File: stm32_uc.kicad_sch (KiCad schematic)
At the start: 28 parts

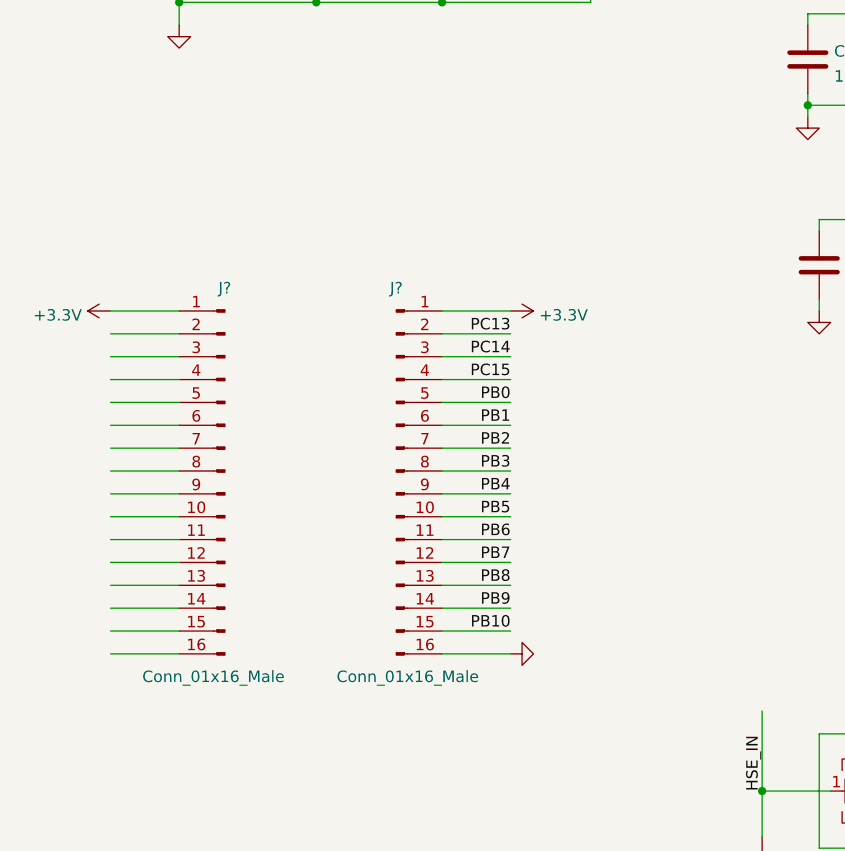
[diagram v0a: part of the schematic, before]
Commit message: finished connectors
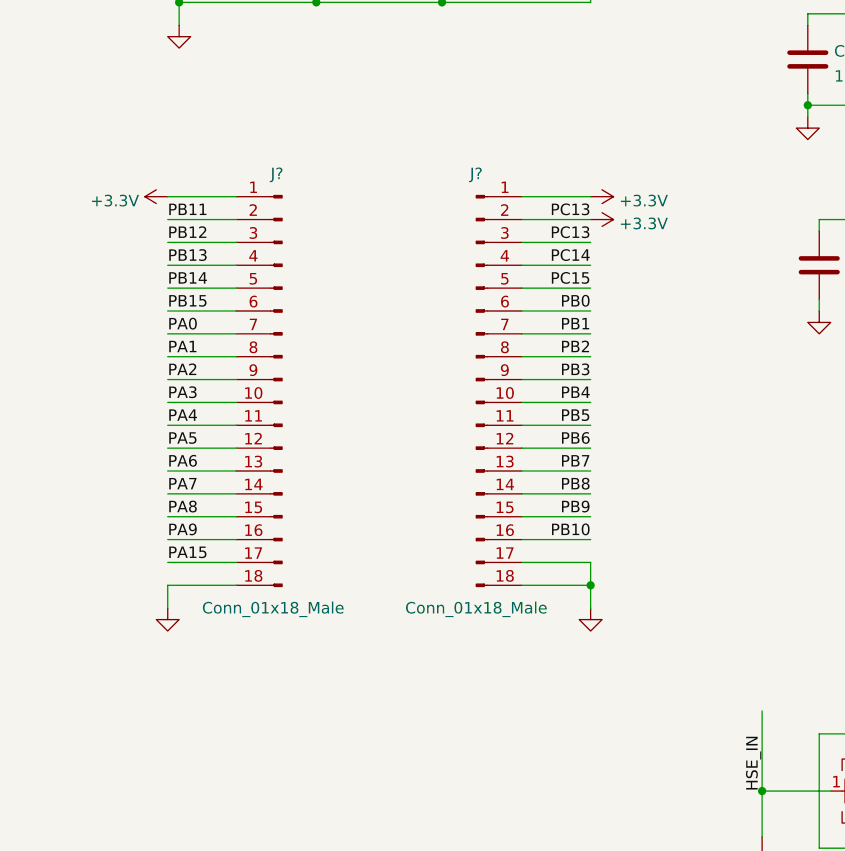
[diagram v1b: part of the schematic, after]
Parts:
- removed J? (x2): Conn_01x16_Male, symbol Connector:Conn_01x16_Male
- added J? (x2): Conn_01x18_Male, symbol Connector:Conn_01x18_Male
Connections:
- net PC13 is gone; now on net +3V3: U?.2 (PC13)
- net +3V3: now also J?.1 (Pin_1), J?.1 (Pin_1), J?.2 (Pin_2), J?.3 (Pin_3)
- net GND: now also J?.17 (Pin_17), J?.18 (Pin_18), J?.18 (Pin_18)
- net PA0: now also J?.7 (Pin_7)
- net PA1: now also J?.8 (Pin_8)
- net PA15: now also J?.17 (Pin_17)
- net PA2: now also J?.9 (Pin_9)
- net PA3: now also J?.10 (Pin_10)
- net PA4: now also J?.11 (Pin_11)
- net PA5: now also J?.12 (Pin_12)
- net PA6: now also J?.13 (Pin_13)
- net PA7: now also J?.14 (Pin_14)
- net PA8: now also J?.15 (Pin_15)
- net PA9: now also J?.16 (Pin_16)
- net PB0: now also J?.6 (Pin_6)
- net PB1: now also J?.7 (Pin_7)
- net PB10: now also J?.16 (Pin_16)
- net PB11: now also J?.2 (Pin_2)
- net PB12: now also J?.3 (Pin_3)
- net PB13: now also J?.4 (Pin_4)
- net PB14: now also J?.5 (Pin_5)
- net PB15: now also J?.6 (Pin_6)
- net PB2: now also J?.8 (Pin_8)
- net PB3: now also J?.9 (Pin_9)
- net PB4: now also J?.10 (Pin_10)
- net PB5: now also J?.11 (Pin_11)
- net PB6: now also J?.12 (Pin_12)
- net PB7: now also J?.13 (Pin_13)
- net PB8: now also J?.14 (Pin_14)
- net PB9: now also J?.15 (Pin_15)
- net PC14: now also J?.4 (Pin_4)
- net PC15: now also J?.5 (Pin_5)

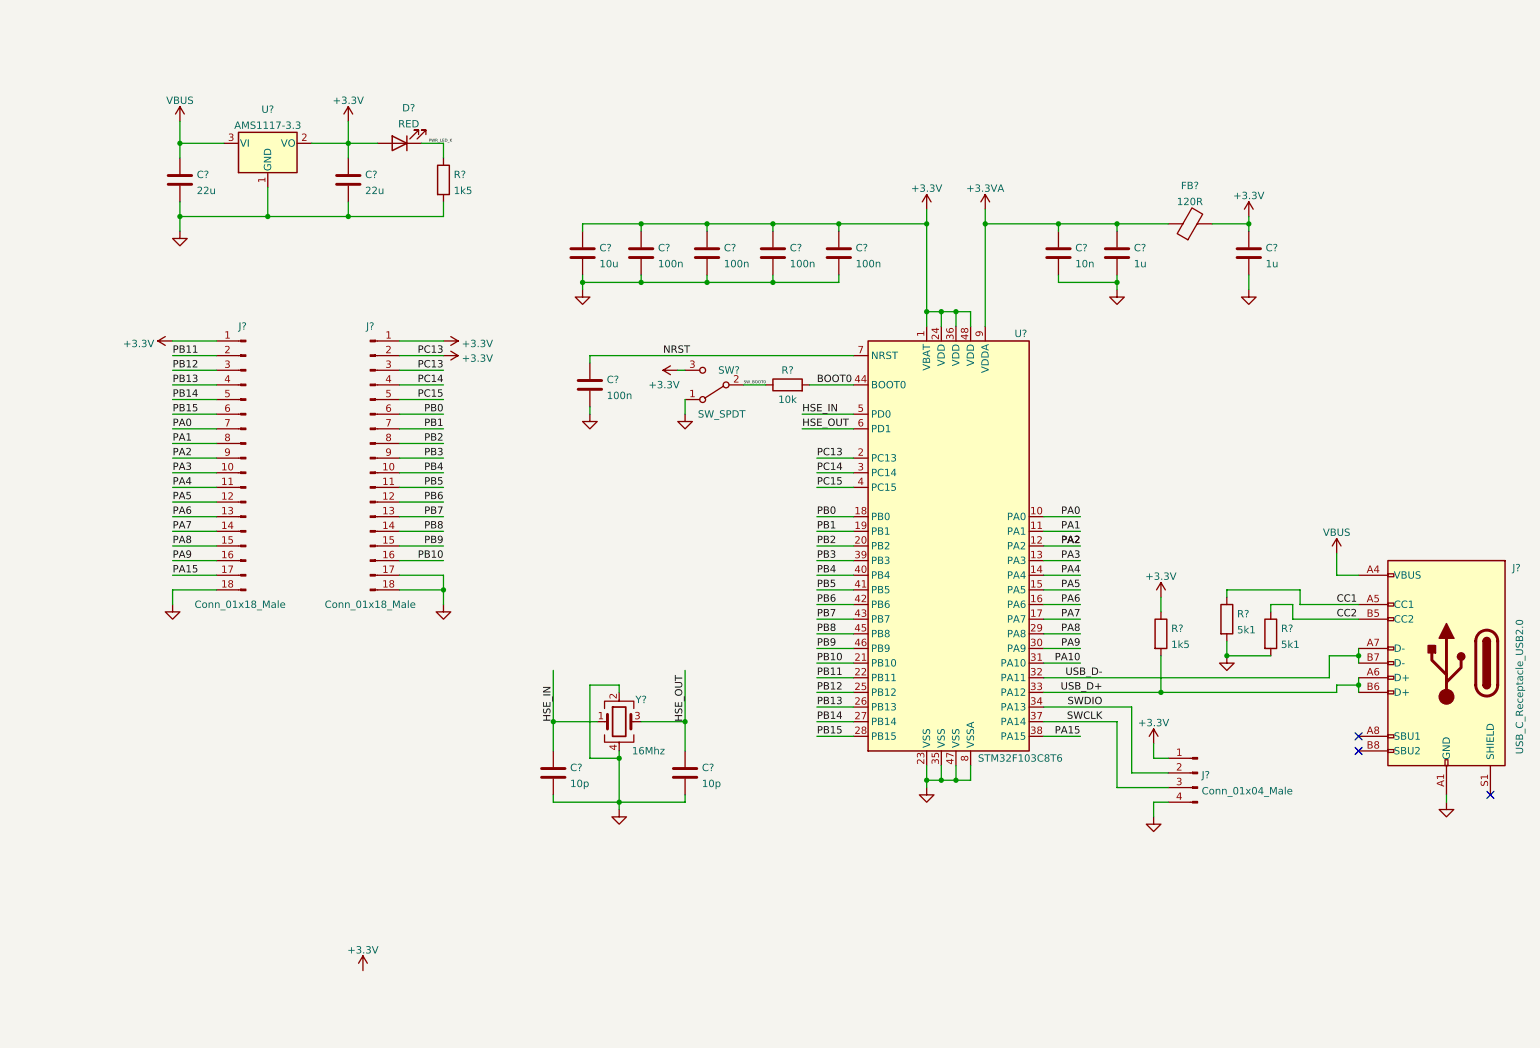
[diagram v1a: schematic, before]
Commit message: started anotating schematic
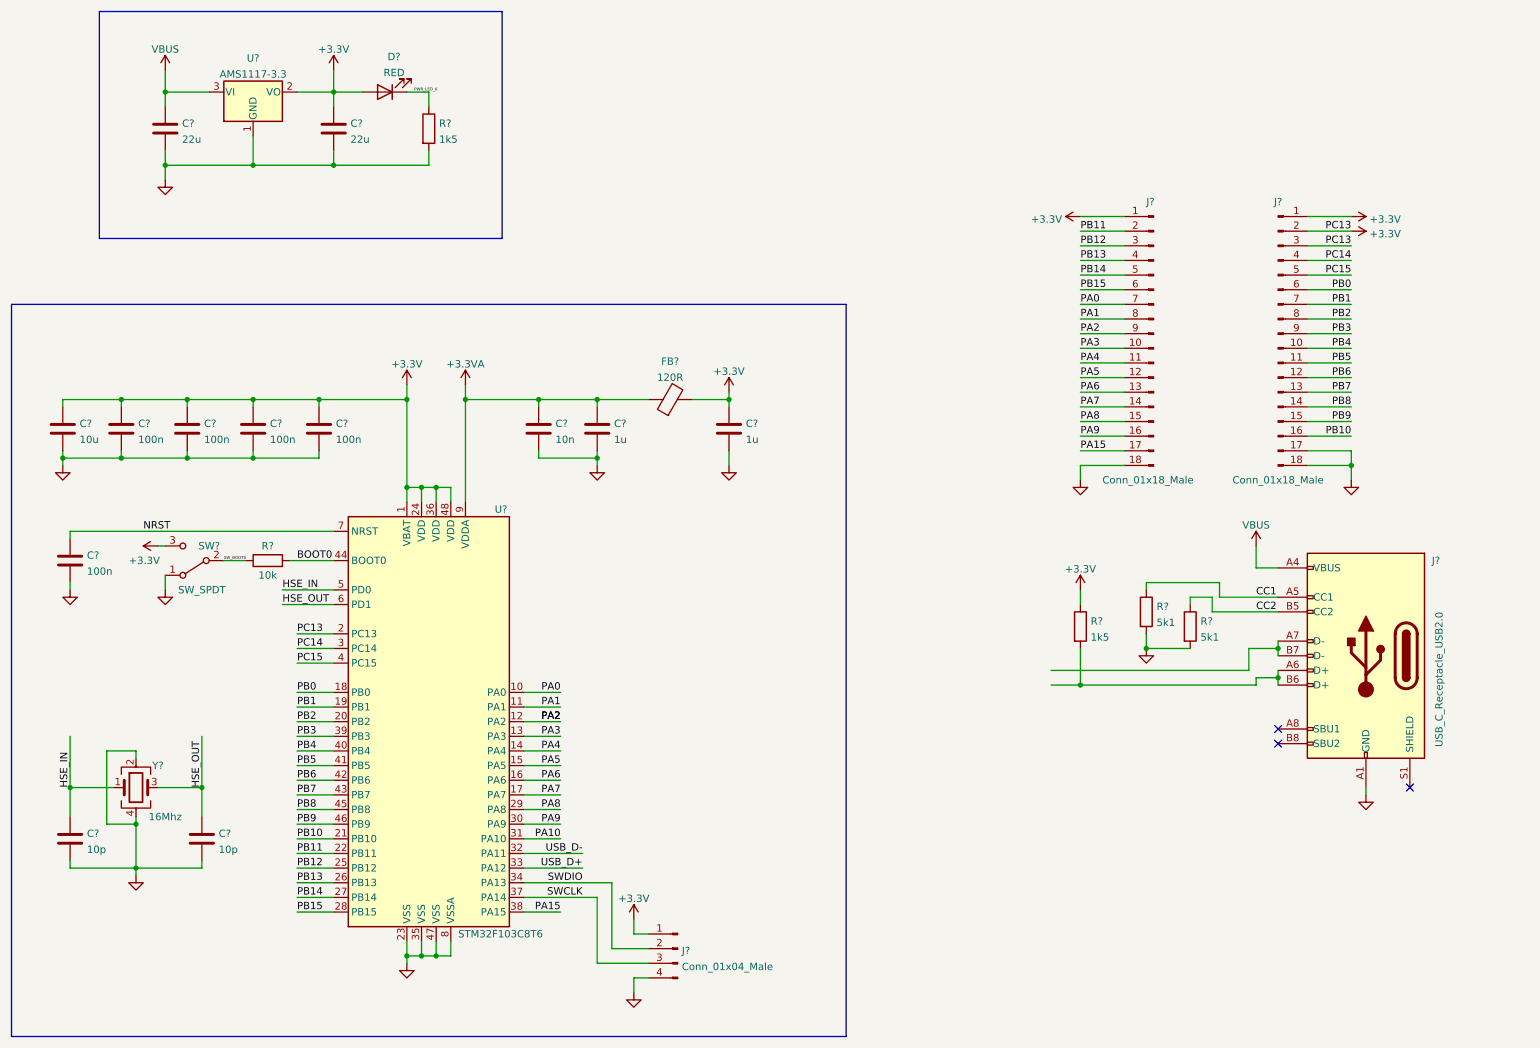
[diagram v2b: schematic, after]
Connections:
- net USB_D+: no longer J?.A6 (D+), J?.B6 (D+), R?.2
- net USB_D-: no longer J?.A7 (D-), J?.B7 (D-)
- new net: J?.A6 (D+), J?.B6 (D+), R?.2
- new net: J?.A7 (D-), J?.B7 (D-)
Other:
- moved on the sheet: C?, D?, FB?, J?, R?, SW?, U?, Y?
